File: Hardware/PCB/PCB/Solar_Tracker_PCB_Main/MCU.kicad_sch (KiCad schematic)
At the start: 1 part, among them IC1 ESP32-S3-WROOM-1-N4R8

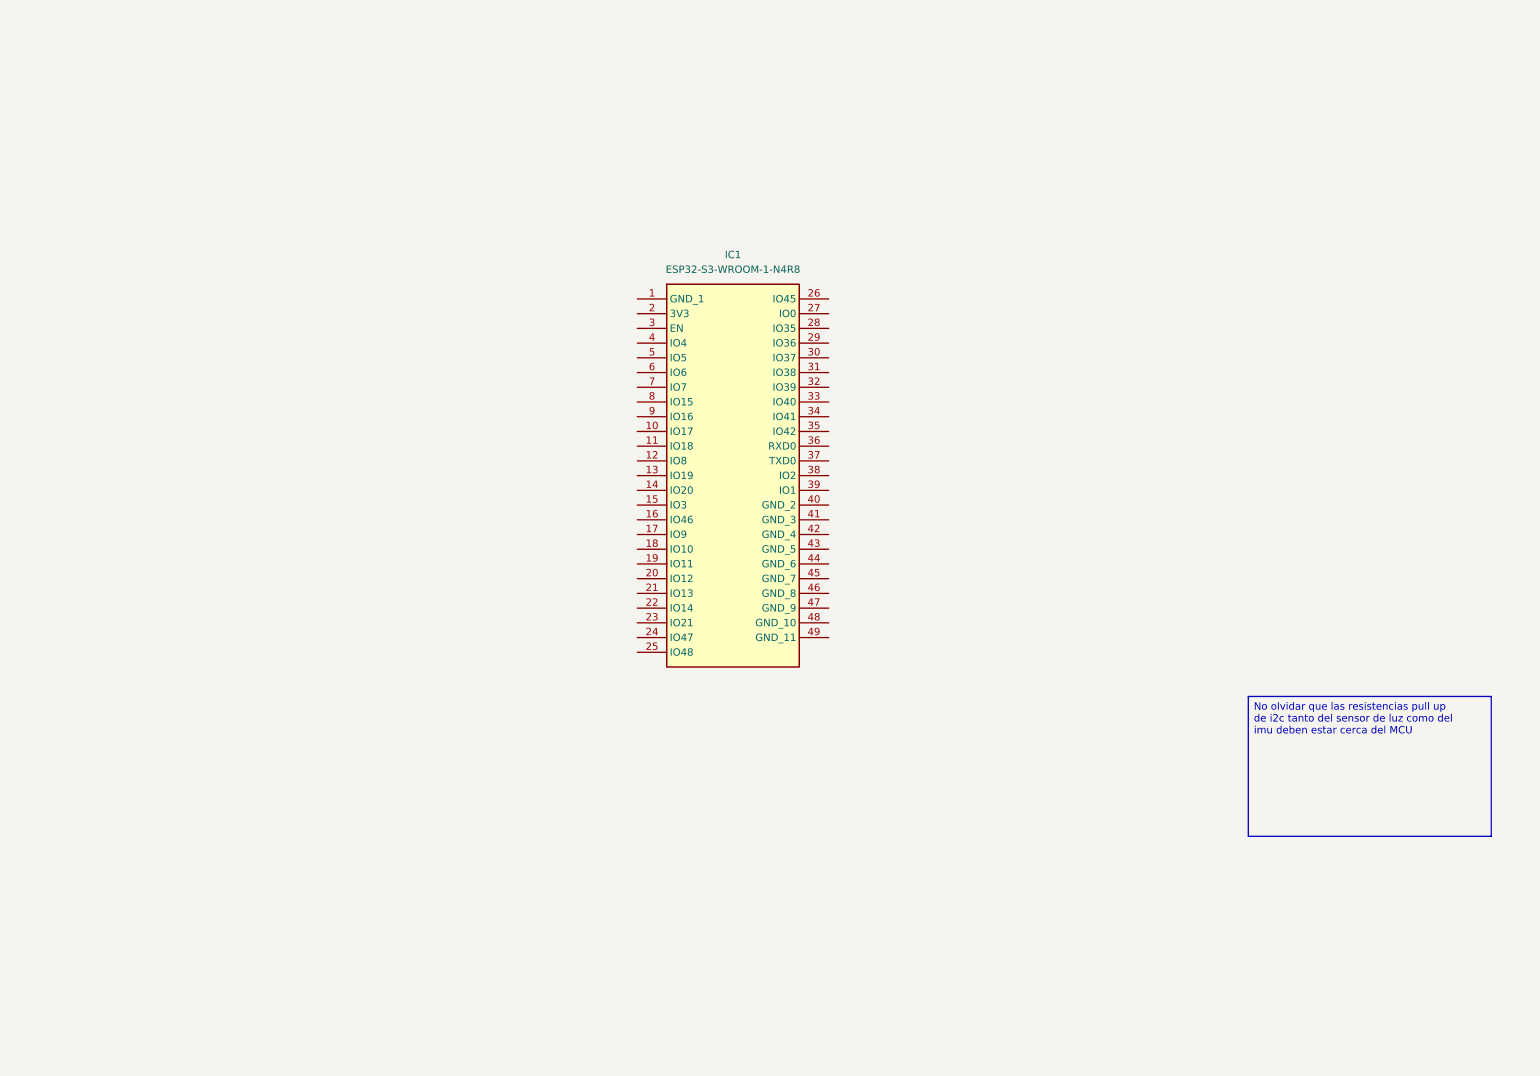
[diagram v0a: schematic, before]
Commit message: actualizacion de pcb
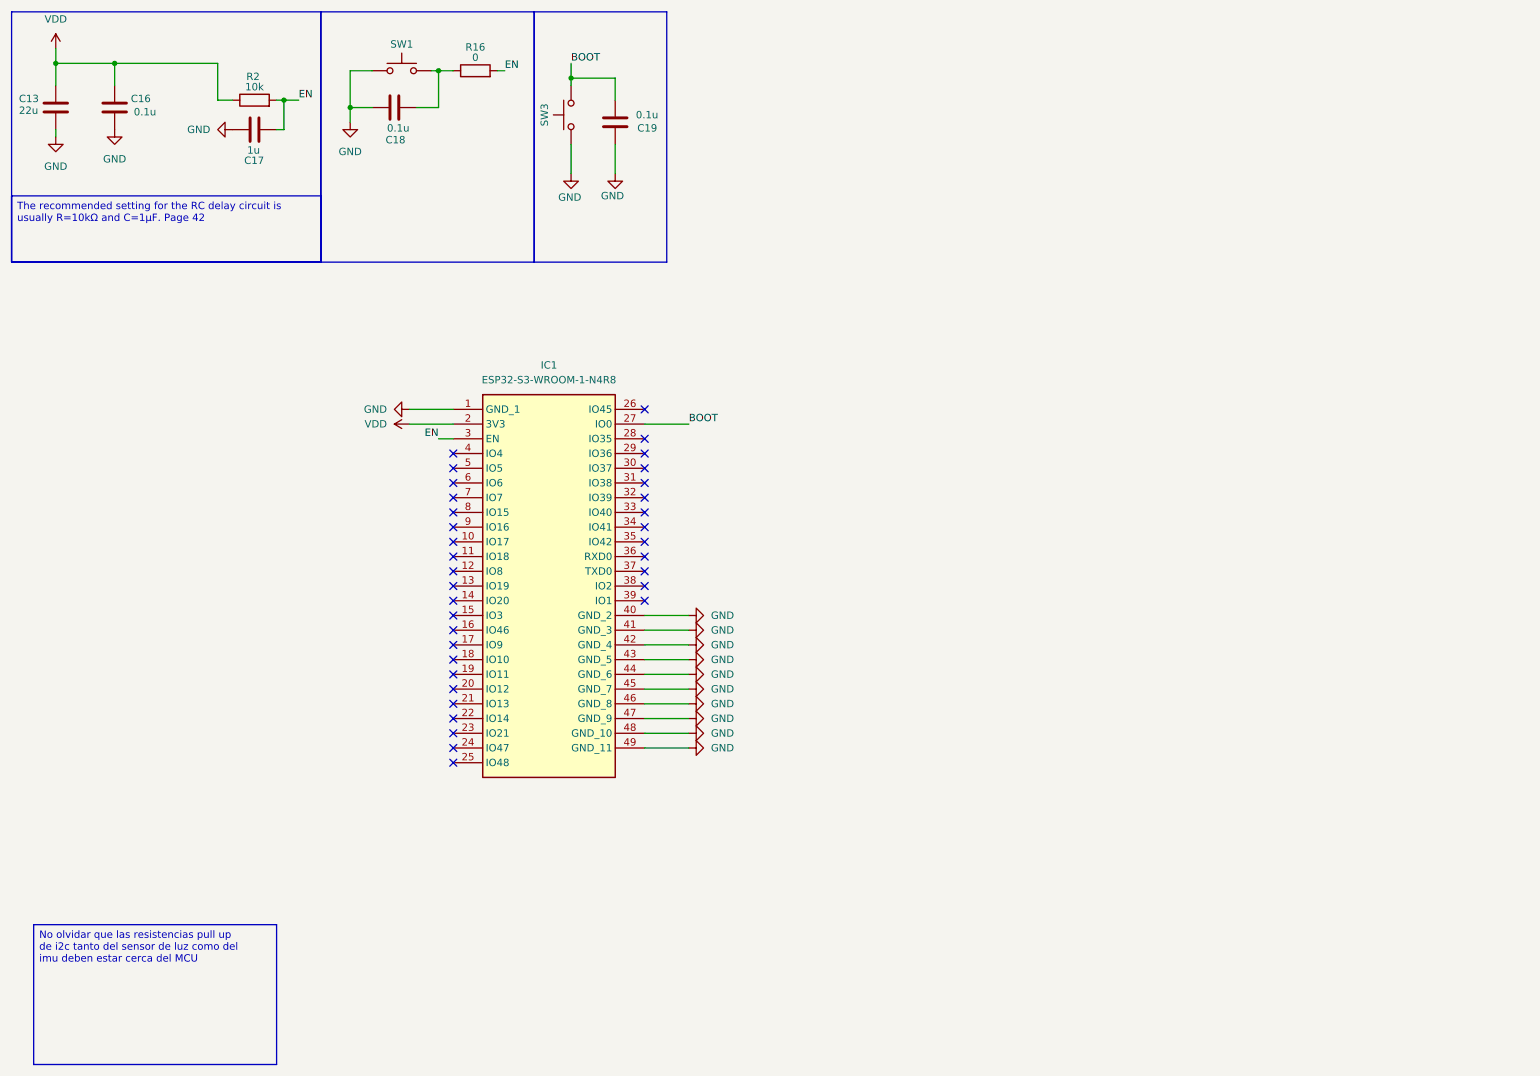
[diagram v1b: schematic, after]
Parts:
- added C13: 22u, symbol Device:C
- added C16, C18, C19: 0.1u, symbol Device:C
- added C17: 1u, symbol Device:C
- added R16: 0, symbol Device:R
- added R2: 10k, symbol Device:R
- added SW1, SW3: ~, symbol Switch:SW_MEC_5G
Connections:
- net GND: now reaches IC1.1 (GND_1)
- net GND: now also IC1.40 (GND_2), IC1.41 (GND_3), IC1.42 (GND_4), IC1.43 (GND_5), IC1.44 (GND_6), IC1.45 (GND_7), IC1.46 (GND_8), IC1.47 (GND_9), IC1.48 (GND_10), IC1.49 (GND_11), C13.2, C16.2, C17.2, C18.2, C19.2, SW1.1 (A), SW1.2 (A), SW3.1 (A), SW3.2 (A)
- net VDD: now reaches IC1.2 (3V3)
- net VDD: now also C13.1, C16.1, R2.1
- net BOOT: now reaches IC1.27 (IO0)
- net BOOT: now also C19.1, SW3.3 (B), SW3.4 (B)
- net EN: now reaches IC1.3 (EN)
- net EN: now also C17.1, R16.2, R2.2
- new net: C18.1, R16.1, SW1.3 (B), SW1.4 (B)
- no-connect marks 0 -> 35
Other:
- moved on the sheet: IC1
